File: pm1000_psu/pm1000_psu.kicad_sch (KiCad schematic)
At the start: 42 parts, among them J3 Screw_Terminal_01x05, U1 LM317_TO-220, U2 LM317_TO-220, U3 LM317_TO-220

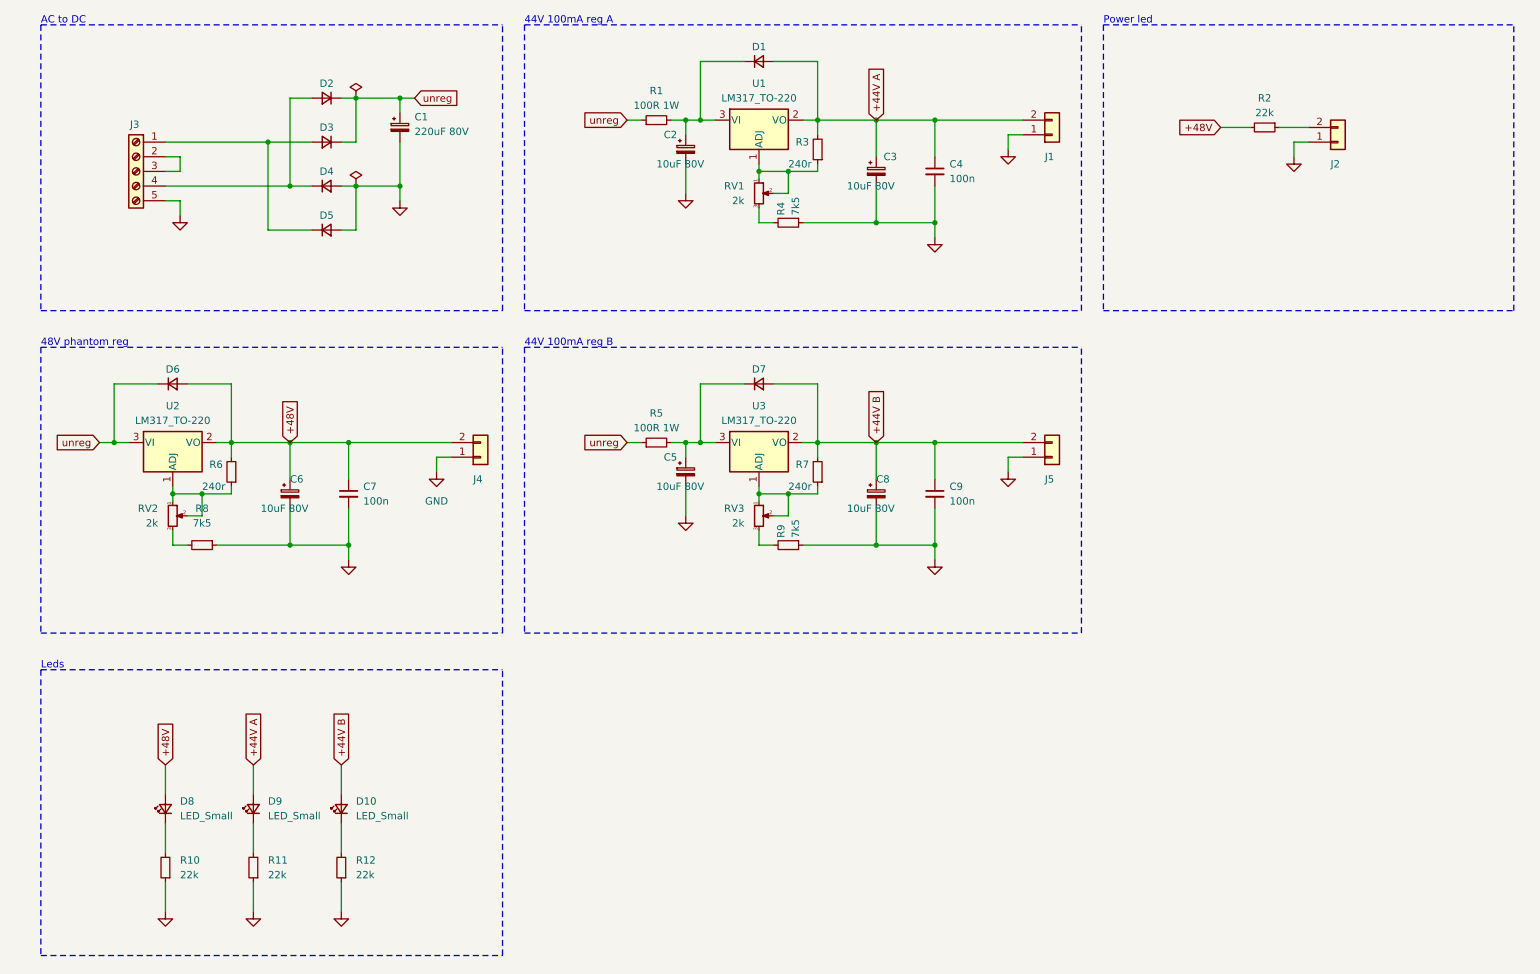
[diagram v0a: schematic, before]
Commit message: clean up project structure, organize psu silkscreen
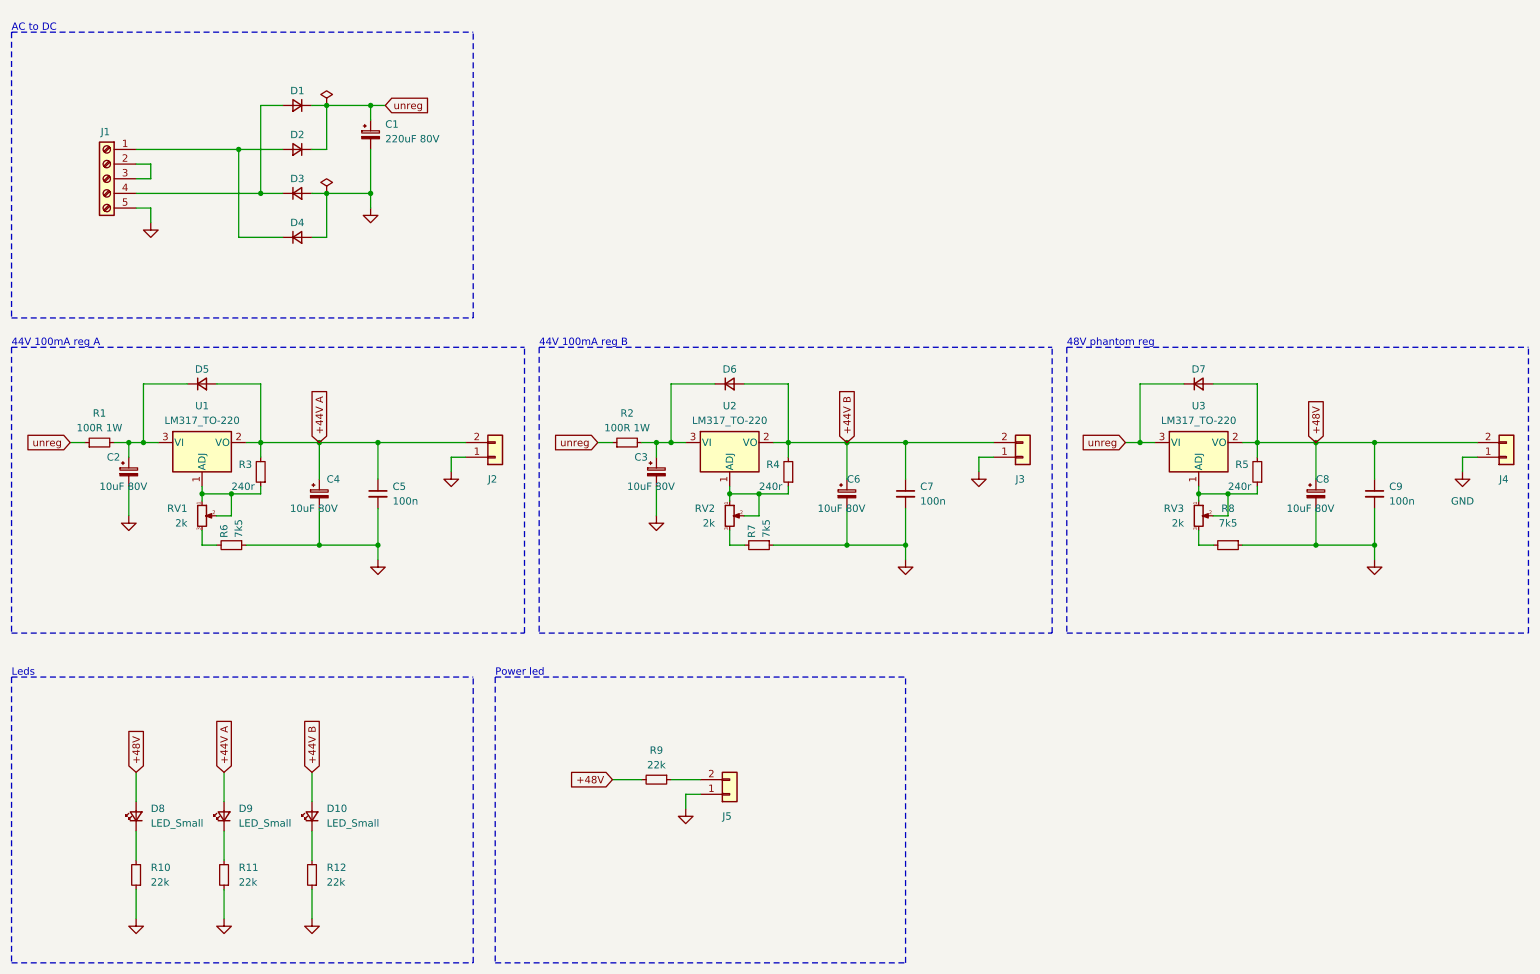
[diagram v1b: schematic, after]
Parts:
- renumbered C5 to C3, C3 to C4, C4 to C5, C8 to C6, C9 to C7, C6 to C8, C7 to C9, D2 to D1, D3 to D2, D4 to D3, D5 to D4, D1 to D5, D7 to D6, D6 to D7, J3 to J1, J1 to J2, J5 to J3, J2 to J5, R5 to R2, R7 to R4, R6 to R5, R4 to R6, R9 to R7, R2 to R9, RV3 to RV2, RV2 to RV3, U3 to U2, U2 to U3
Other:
- moved on the sheet: C1, C2, C3, C4, C5, C6, C7, C8, C9, D1, D10, D2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
